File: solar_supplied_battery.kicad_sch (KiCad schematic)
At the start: 16 parts, among them J1 Conn_01x02_Pin, J2 Conn_01x02_Pin, J3 Conn_01x02_Pin, J4 Conn_01x02_Pin, Q1 2N7002, U1 AP3015AKTR-G1

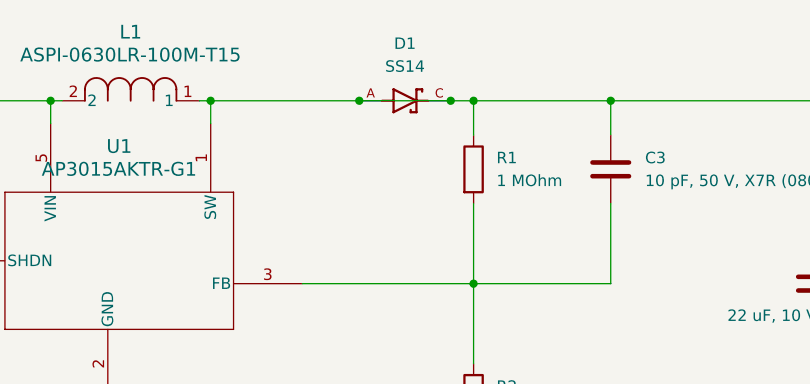
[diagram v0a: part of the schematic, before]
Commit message: starting routes
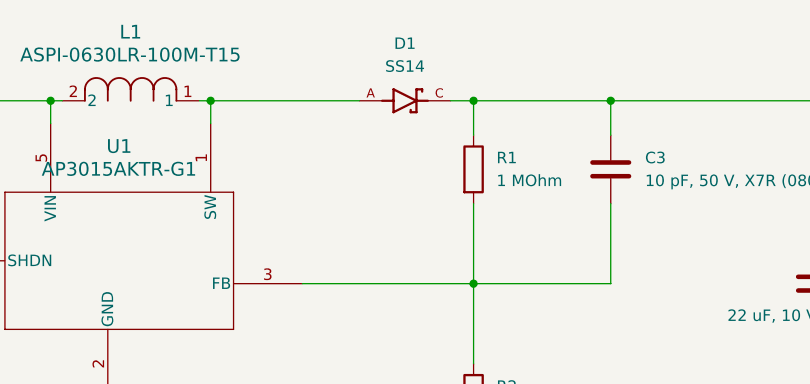
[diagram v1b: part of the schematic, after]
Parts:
- J1, J2: footprint Connector_PinHeader_2.54mm:PinHeader_1x02_P2.54mm_Vertical -> TerminalBlock:TerminalBlock_MaiXu_MX126-5.0-02P_1x02_P5.00mm
- J4: footprint Connector_PinHeader_2.54mm:PinHeader_1x02_P2.54mm_Horizontal -> TerminalBlock:TerminalBlock_MaiXu_MX126-5.0-02P_1x02_P5.00mm
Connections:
- net OUT_P: no longer D1.A, L1.1, U1.1 (SW)
- new net: D1.A, L1.1, U1.1 (SW)
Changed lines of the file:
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@@
-	)
-	(junction
-		(at 176.53 91.44)
-		(diameter 0)
-		(color 0 0 0 0)
-	)
-	(junction
-		(at 166.37 91.44)
-		(diameter 0)
-		(color 0 0 0 0)
 	)
 	(junction
@@
 		(pts
 			(xy 115.57 91.44) (xy 115.57 119.38)
-		)
-		(stroke
-			(width 0)
-			(type default)
-		)
-	)
-	(wire
-		(pts
-			(xy 166.37 91.44) (xy 176.53 91.44)
 		)
 		(stroke
@@
 			)
 		)
-		(property "Footprint" "Connector_PinHeader_2.54mm:PinHeader_1x02_P2.54mm_Vertical"
+		(property "Footprint" "TerminalBlock:TerminalBlock_MaiXu_MX126-5.0-02P_1x02_P5.00mm"
 			(at 82.55 106.68 0)
 			(hide yes)
@@
 			)
 		)
-		(property "Footprint" "Connector_PinHeader_2.54mm:PinHeader_1x02_P2.54mm_Vertical"
+		(property "Footprint" "TerminalBlock:TerminalBlock_MaiXu_MX126-5.0-02P_1x02_P5.00mm"
 			(at 234.95 110.49 0)
 			(hide yes)
@@
 			)
 		)
-		(property "Footprint" "Connector_PinHeader_2.54mm:PinHeader_1x02_P2.54mm_Horizontal"
+		(property "Footprint" "TerminalBlock:TerminalBlock_MaiXu_MX126-5.0-02P_1x02_P5.00mm"
 			(at 63.5 111.76 0)
 			(hide yes)
